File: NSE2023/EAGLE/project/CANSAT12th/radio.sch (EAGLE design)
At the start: 25 parts, among them CN1 DM3AT

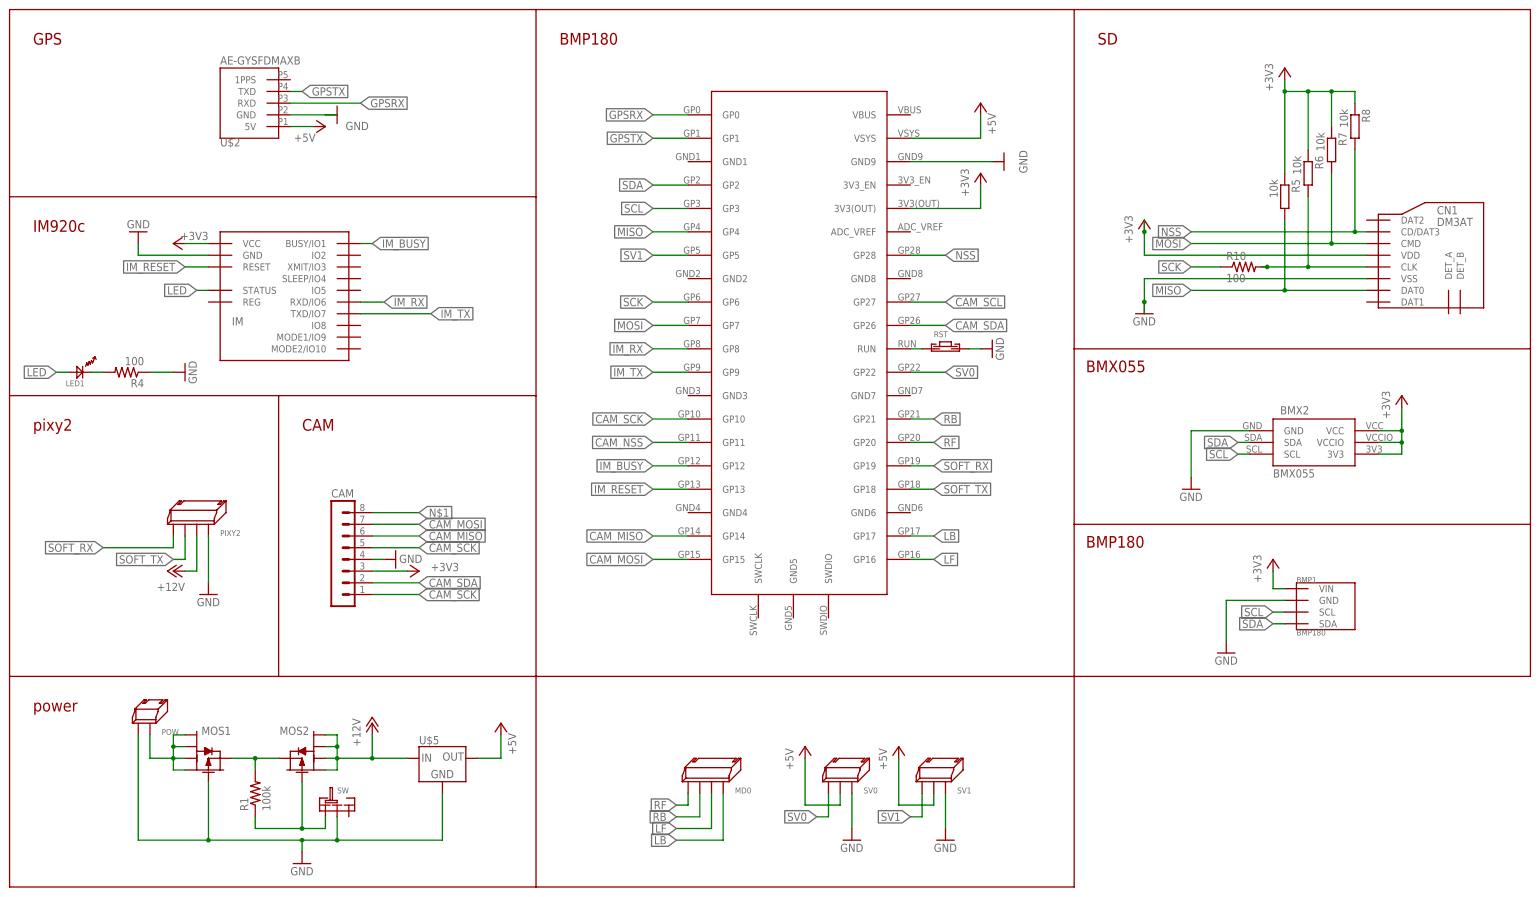
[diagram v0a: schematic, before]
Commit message: add
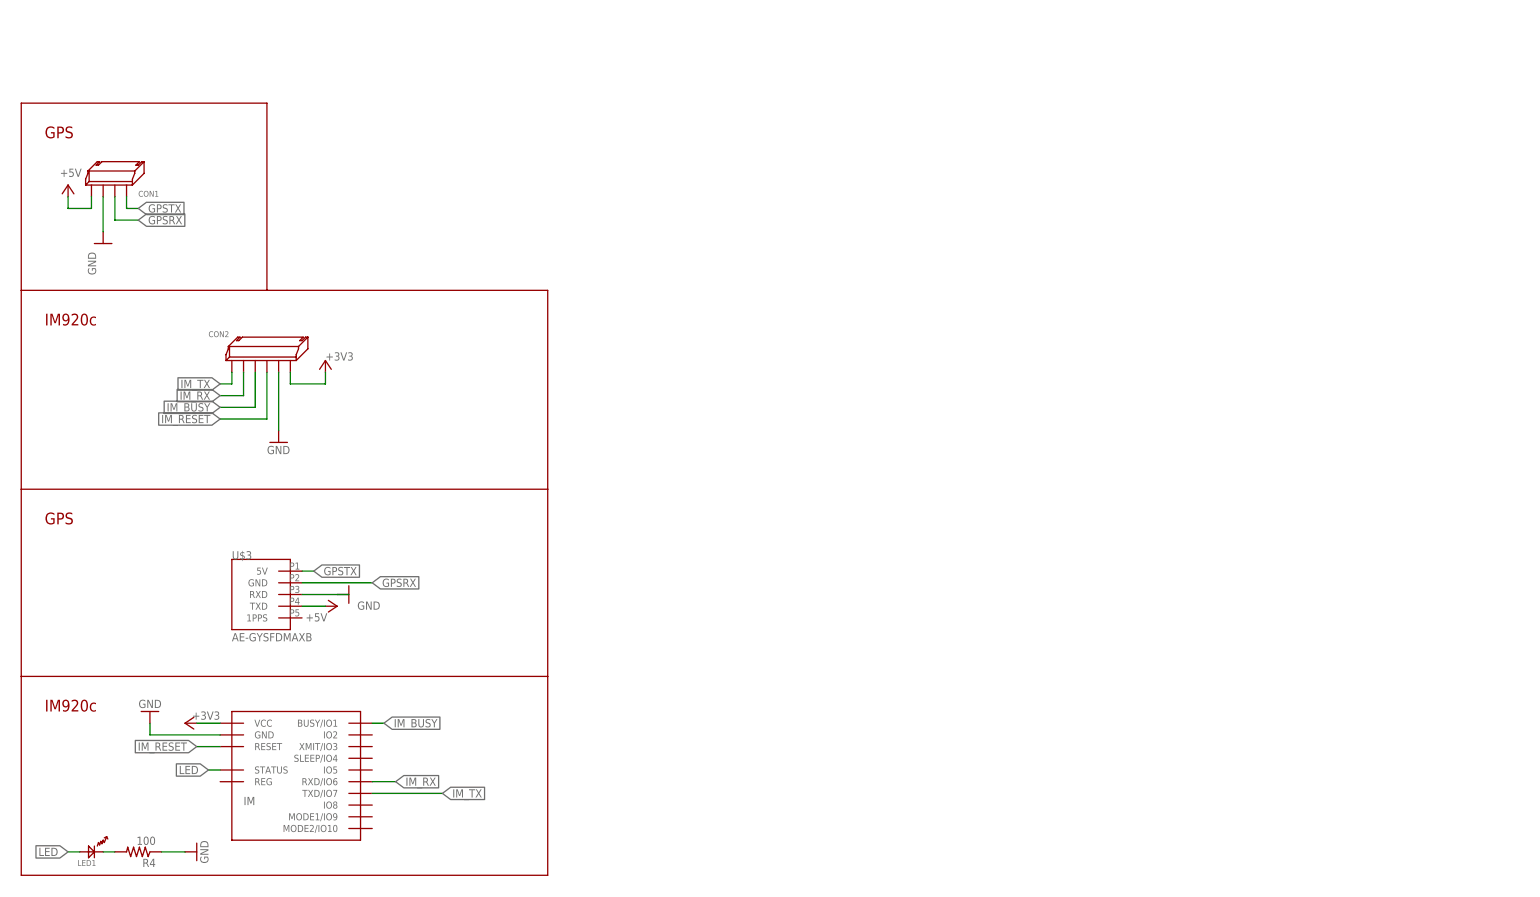
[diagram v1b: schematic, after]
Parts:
- removed BMP1: BMP180, BMP180:BMP180
- removed BMX2: BMX055, BMX055:BMX055
- removed CAM: (no value), con-lstb:MA08-1
- removed CN1: DM3AT, microSD:DM3AT
- removed MD0, PIXY2: (no value), XR Connector:4PIN_SIDE
- removed MOS1, MOS2: (no value), Chip MOSFET:PCH_SSM6J808R
- removed POW: (no value), XR Connector:2PIN_SIDE
- removed R1: 100k, rcl:R-US_R0603
- removed R10: 100, rcl:R-US_R0603
- removed R5, R6, R7, R8: 10k, rcl:R-EU_R0603
- removed RST: (no value), Tact switch:TVAF06-A020B-R
- removed SV0, SV1: (no value), XR Connector:3PIN_SIDE
- removed SW: SRIDE_SWITCH, Sride Switch:SRIDE_SWITCH
- removed U$1: RASPBERRYPIPICO, Raspberry Pi Pico:RASPBERRYPIPICO
- removed U$2: AE-GYSFDMAXB, AE-GYSFDMAXB:AE-GYSFDMAXB
- removed U$5: LT1117-5, LT1117:LT1117-5
- added CON1: (no value), XR Connector:4PIN_SIDE
- added CON2: (no value), XR Connector:6PIN_SIDE
- added U$3: AE-GYSFDMAXB, AE-GYSFDMAXB:AE-GYSFDMAXB
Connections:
- removed net +12V: MOS2.1, MOS2.2, MOS2.5, MOS2.6, PIXY2.P$3, U$5.IN
- removed net CAM_MISO: CAM.6, U$1.GP14
- removed net CAM_MOSI: CAM.7, U$1.GP15
- removed net CAM_NSS: U$1.GP11
- removed net CAM_SCK: CAM.1, CAM.5, U$1.GP10
- removed net CAM_SCL: U$1.GP27
- removed net CAM_SDA: CAM.2, U$1.GP26
- removed net LB: MD0.P$4, U$1.GP17
- removed net LF: MD0.P$3, U$1.GP16
- removed net MISO: CN1.DAT0, R5.2, U$1.GP4
- removed net MOSI: CN1.CMD, R7.2, U$1.GP7
- removed net N$1: CAM.8
- removed net N$2: RST.P$1, U$1.RUN
- removed net N$4: U$1.GND9
- removed net N$6: MOS1.4, MOS2.4, R1.2
- removed net N$7: MOS2.3, R1.1, SW.L
- removed net N$8: MOS1.1, MOS1.2, MOS1.5, MOS1.6, POW.P$1
- removed net NSS: CN1.CD/DAT3, R8.2, U$1.GP28
- removed net RB: MD0.P$1, U$1.GP21
- removed net RF: MD0.P$2, U$1.GP20
- removed net SCK: CN1.CLK, R10.1, R10.2, R6.2, U$1.GP6
- removed net SCL: BMP1.SCL, BMX2.SCL, U$1.GP3
- removed net SDA: BMP1.SDA, BMX2.SDA, U$1.GP2
- removed net SOFT_RX: PIXY2.P$2, U$1.GP19
- removed net SOFT_TX: PIXY2.P$1, U$1.GP18
- removed net SV0: SV0.P$2, U$1.GP22
- removed net SV1: SV1.P$2, U$1.GP5
- net +3V3: now also CON2.P$6; no longer BMP1.VIN, BMX2.3V3, BMX2.VCC, BMX2.VCCIO, CAM.3, CN1.VDD, R5.1, R6.1, R7.1, R8.1, U$1.3V3(OUT)
- net +5V: now also CON1.P$2, U$3.TXD; no longer SV0.P$1, SV1.P$1, U$1.VSYS, U$2.5V, U$5.OUT
- net GND: now also CON1.P$1, CON2.P$5; no longer BMP1.GND, BMX2.GND, CAM.4, CN1.VSS, MOS1.3, PIXY2.P$4, POW.P$2, RST.P$2, SV0.P$3, SV1.P$3, SW.LR, U$5.GND
- net GND1: now also U$3.RXD; no longer U$2.GND
- net GPSRX: now also CON1.P$3, U$3.GND; no longer U$1.GP0, U$2.RXD
- net GPSTX: now also CON1.P$4, U$3.5V; no longer U$1.GP1, U$2.TXD
- net IM_BUSY: now also CON2.P$3; no longer U$1.GP12
- net IM_RESET: now also CON2.P$4; no longer U$1.GP13
- net IM_RX: now also CON2.P$2; no longer U$1.GP8
- net IM_TX: now also CON2.P$1; no longer U$1.GP9
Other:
- note removed: "BMP180"
- note removed: "BMX055"
- note removed: "CAM"
- note removed: "SD"
- note removed: "pixy2"
- note removed: "power"
- moved on the sheet: IM, LED1, R4
